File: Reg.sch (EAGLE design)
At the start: 25 parts, among them Q1 NPN, Q2 NPN, Q3 PNP, Q4 NPN, Q5 NPN, Q6 NPN, Q8 PNP

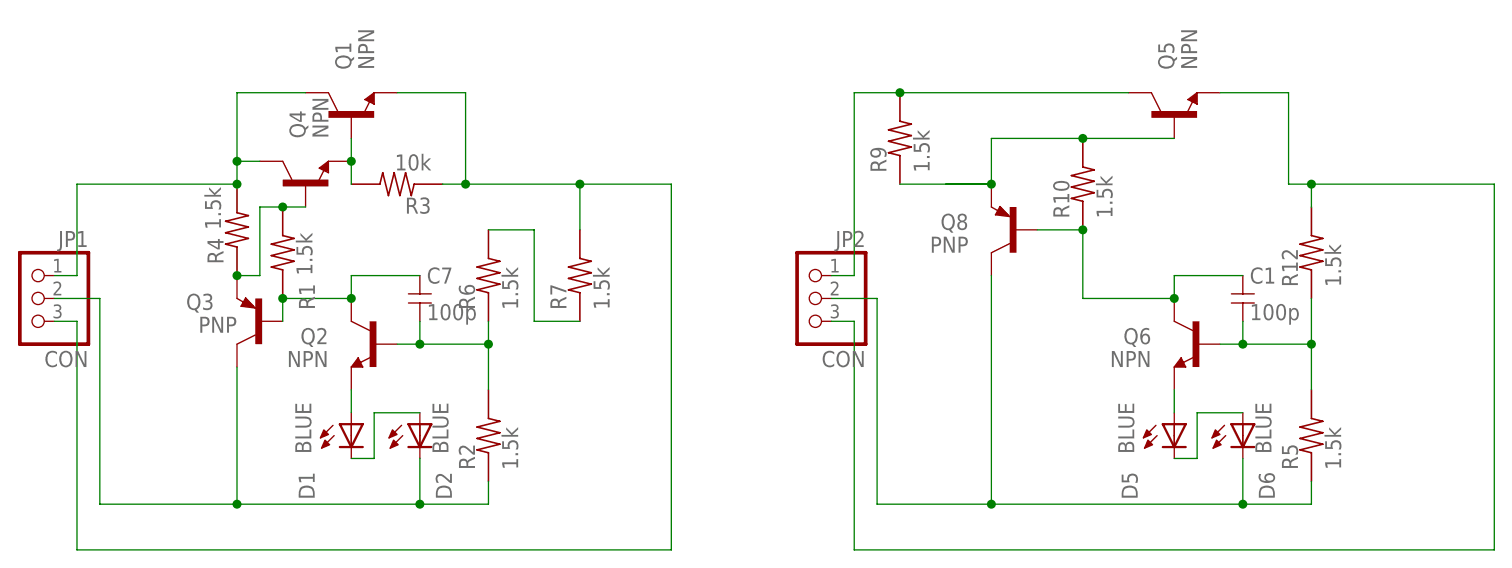
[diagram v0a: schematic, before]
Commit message: LDO ver
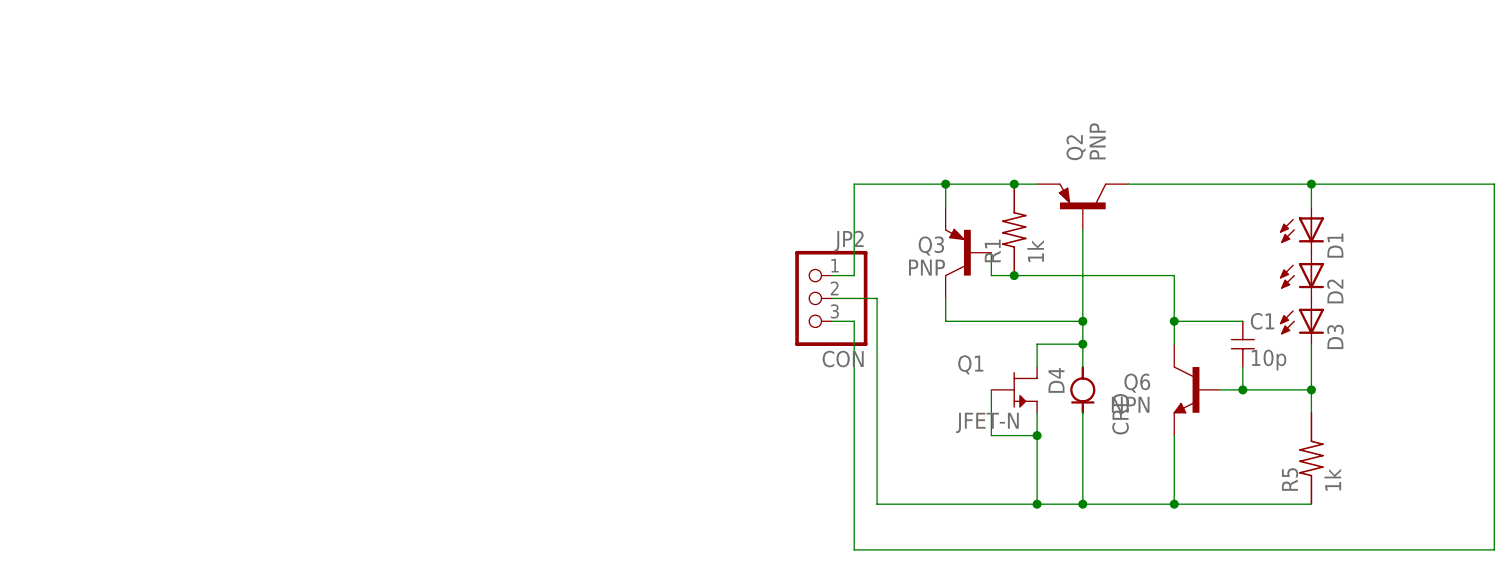
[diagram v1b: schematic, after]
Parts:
- removed C7: 100p, my_rcl:C-1608
- removed D5, D6: BLUE, my_rcl:LED-SMD1608
- removed JP1: CON, pinhead:PINHD-1X3
- removed Q4: NPN, my_ic:NPN2SC3325
- removed Q5: NPN, my_ic:NPN-SOT223
- removed Q8: PNP, my_ic:PNP2SA1313
- removed R10, R12, R2, R4, R6, R7, R9: 1.5k, my_rcl:R-1608
- removed R3: 10k, my_rcl:R-1608
- added D3: (no value), my_rcl:LED-SMD2012
- added D4: CRD, my_rcl:CRD-SMD
- C1: value 100p -> 10p
- D1, D2: value BLUE -> (none); device my_rcl:LED-SMD1608 -> my_rcl:LED-SMD2012
- JP2: device pinhead:PINHD-1X3 -> my_connector:SW-1X3
- Q1: value NPN -> JFET-N; device my_ic:NPN2SC3422-2 -> my_ic:JFET-N
- Q2: value NPN -> PNP; device my_ic:NPN2SC3325 -> my_ic:PNP2SA1359-2
- R1, R5: value 1.5k -> 1k
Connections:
- removed net GND: D2.K, JP1.2, Q3.C, R2.1
- removed net IN: JP1.1, Q1.C, Q4.C, R4.2
- removed net N$1 (its old number): Q3.E, Q4.B, R1.2, R4.1
- removed net N$10: C7.1, Q2.C, Q3.B, R1.1
- removed net N$12: C1.1, Q6.C, Q8.B, R10.1
- removed net N$16: Q5.B, Q8.E, R10.2, R9.1
- removed net N$3: C7.2, Q2.B, R2.2, R6.1
- removed net N$6: Q1.B, Q4.E, R3.2
- removed net N$8: D5.K, D6.A
- removed net N$9: D5.A, Q6.E
- removed net OUT: JP1.3, Q1.E, R3.1, R7.2
- new net N$2: D2.K, D3.A
- net GND1: now also D4.K, Q1.G, Q1.S, Q6.E; no longer D6.K, Q8.C
- net IN1: now also Q2.E, Q3.E, R1.2; no longer Q5.C, R9.2
- net N$13: now also D3.K; no longer R12.1
- net N$4: now also D4.A, Q1.D, Q2.B, Q3.C; no longer D1.A, Q2.E
- net N$5: now also C1.1, Q3.B, Q6.C, R1.1; no longer R6.2, R7.1
- net OUT1: now also D1.A, Q2.C; no longer Q5.E, R12.2
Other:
- moved on the sheet: C1, D1, D2, Q3, Q6, R1, R5
